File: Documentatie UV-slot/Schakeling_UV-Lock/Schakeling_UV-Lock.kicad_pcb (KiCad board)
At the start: 2 copper layers, 7.6 x 1.2 mm, 21 parts, among them Q1 BC817

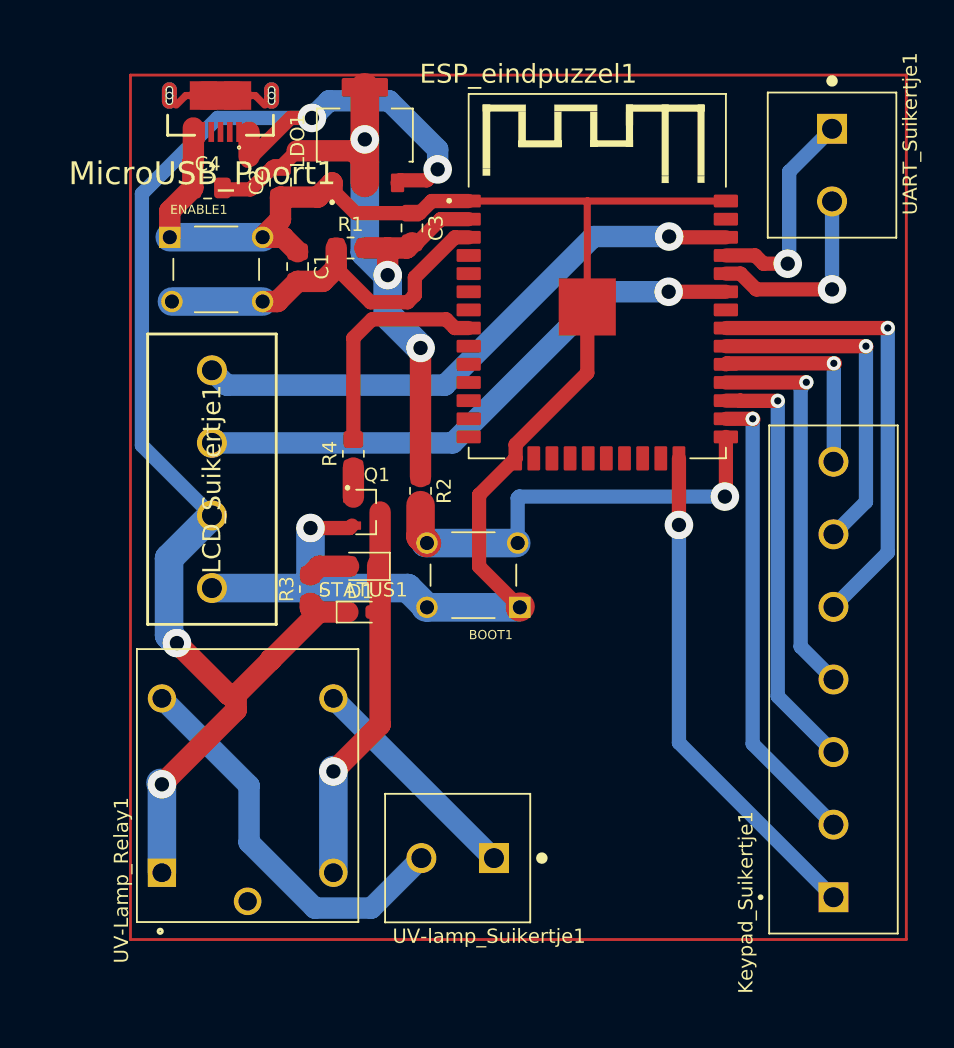
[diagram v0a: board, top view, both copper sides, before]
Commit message: Veel nieuwe aanpassing in de Kicad files ( en ook een paar in de code)
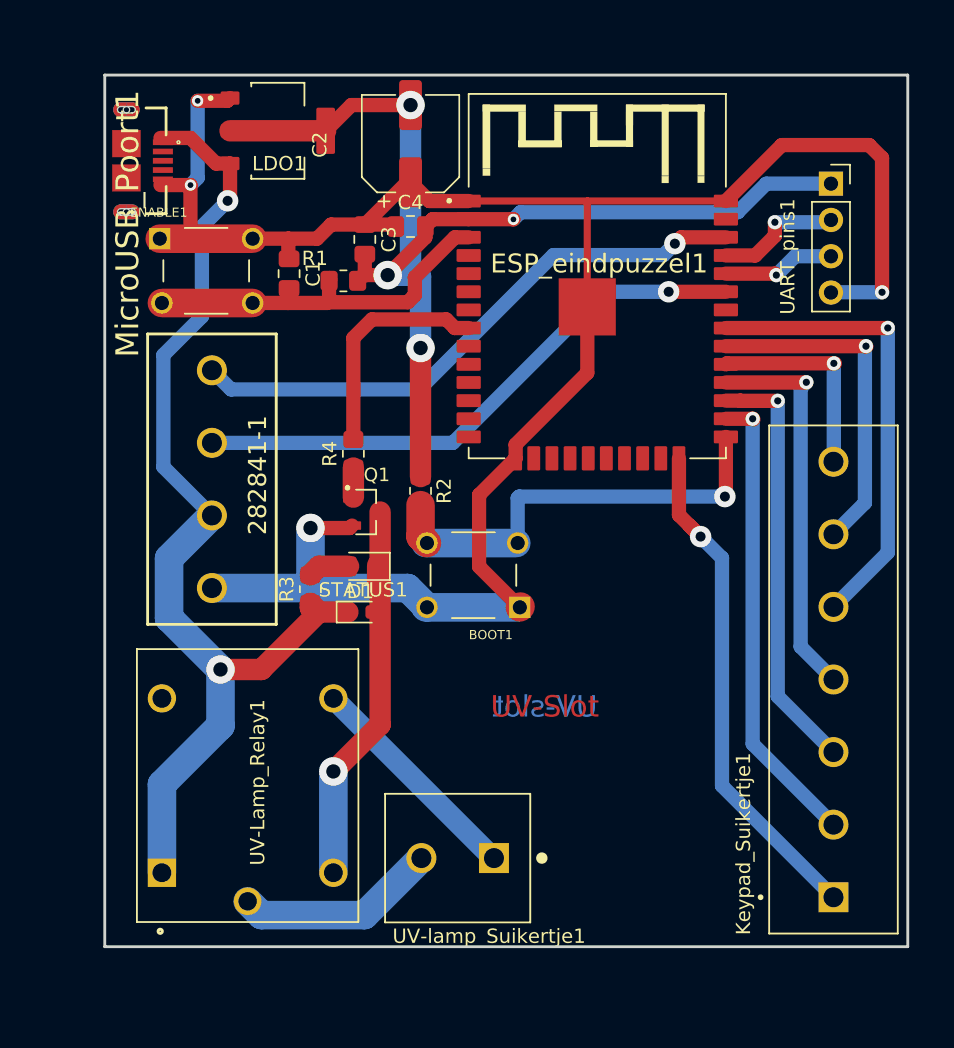
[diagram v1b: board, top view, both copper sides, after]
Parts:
- removed UART_Suikertje1: 282841-2, components:TE_282841-2
- added UART_pins1: Conn_01x04_Female, Connector_PinSocket_2.54mm:PinSocket_1x04_P2.54mm_Vertical, F.Cu at (119.5, 80.2)
- C2: footprint Capacitor_SMD:C_0805_2012Metric_Pad1.18x1.45mm_HandSolder -> Capacitor_SMD:CP_Elec_6.3x7.7
- moved C4 14.5 mm to (90.1, 83.2)
- moved C2 9.49 mm to (90.1, 77.4)
- moved MicroUSB_Poort1 8.01 mm to (70.2, 78.6), turned to -90 degrees
- moved LDO1 6.09 mm to (80.8, 76.5), turned to 0 degrees
- moved C3 3.40 mm to (86.9, 84.1)
- moved R1 2.35 mm to (85.4, 87.0)
- moved C1 0.78 mm to (81.6, 86.5)
- moved ENABLE1 0.71 mm to (75.8, 86.3)
- renumbered LCD_Suikertje1 to 282841-1
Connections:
- ESP_eindpuzzel1 pad 34: Net-(ESP_eindpuzzel1-Pad34) -> RX
- ESP_eindpuzzel1 pad 35: Net-(ESP_eindpuzzel1-Pad35) -> TX
- UV-Lamp_Relay1 pad COM: unconnected-(UV-Lamp_Relay1-PadCOM) -> Net-(UV-Lamp_Relay1-PadCOM)
- UV-Lamp_Relay1 pad NC: Net-(UV-Lamp_Relay1-PadNC) -> unconnected-(UV-Lamp_Relay1-PadNC)
- UV-lamp_Suikertje1 pad 2: Net-(UV-Lamp_Relay1-PadNC) -> Net-(UV-Lamp_Relay1-PadCOM)
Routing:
- net GND: track 116.2 -> 152.1 mm, vias 1 -> 4
- net 5V: track 103.7 -> 74.9 mm, vias 4 -> 2
- net 3.3V: track 53.0 -> 81.2 mm, vias 3 -> 4
- net Net-(UV-Lamp_Relay1-PadNC): track 28.0 -> 0.00 mm
- net Net-(ESP_eindpuzzel1-Pad35): track 15.3 -> 0.00 mm, vias 1 -> 0
- net Net-(UV-Lamp_Relay1-PadCOM): track 0.00 -> 14.2 mm
- net Net-(ESP_eindpuzzel1-Pad34): track 14.0 -> 0.00 mm, vias 1 -> 0
- net TX: track 0.00 -> 8.94 mm, vias 0 -> 1
- net RX: track 0.00 -> 7.95 mm, vias 0 -> 1
- net unconnected-(MicroUSB_Poort1-Pad6): track 6.75 -> 0.00 mm
- net IO2: track 35.2 -> 36.3 mm
- added copper zone on B.Cu, net GND
- added copper zone on F.Cu, net GND
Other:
- board size 7.6 x 1.2 mm -> 56.2 x 61 mm
- board text added: "UV-Slot"
- board text added: "UV-slot"
